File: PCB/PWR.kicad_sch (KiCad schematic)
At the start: 21 parts, among them U3 LT8610

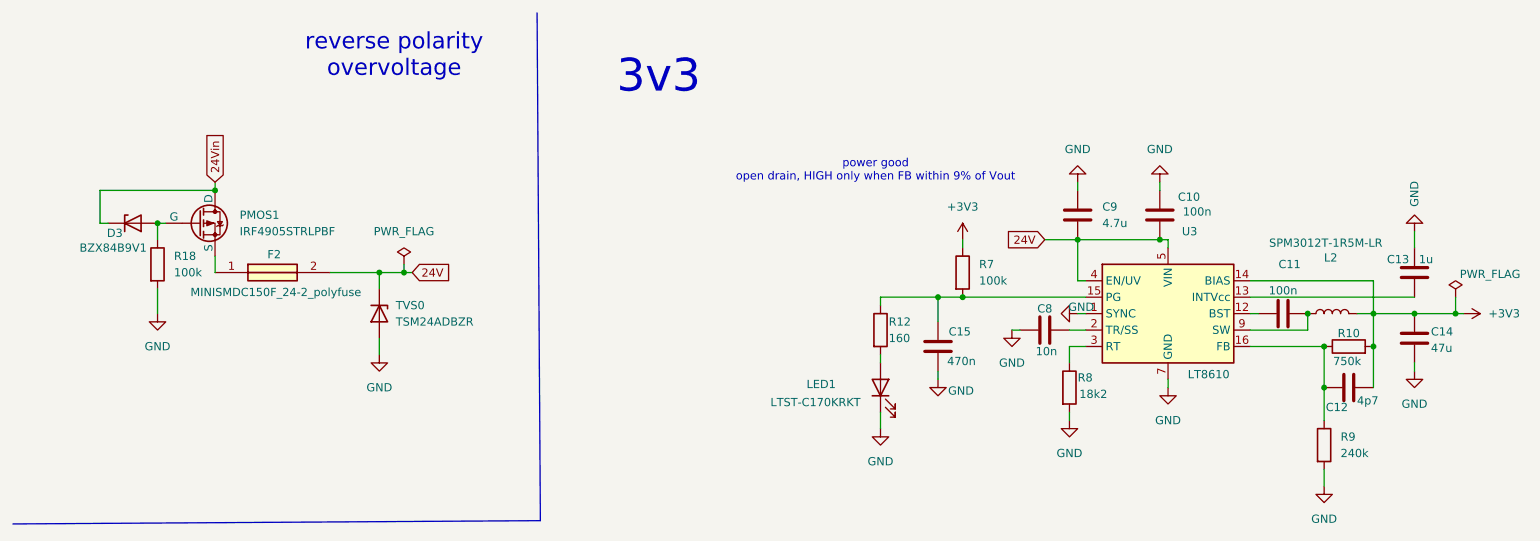
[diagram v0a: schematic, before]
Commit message: pcb version ready for final check
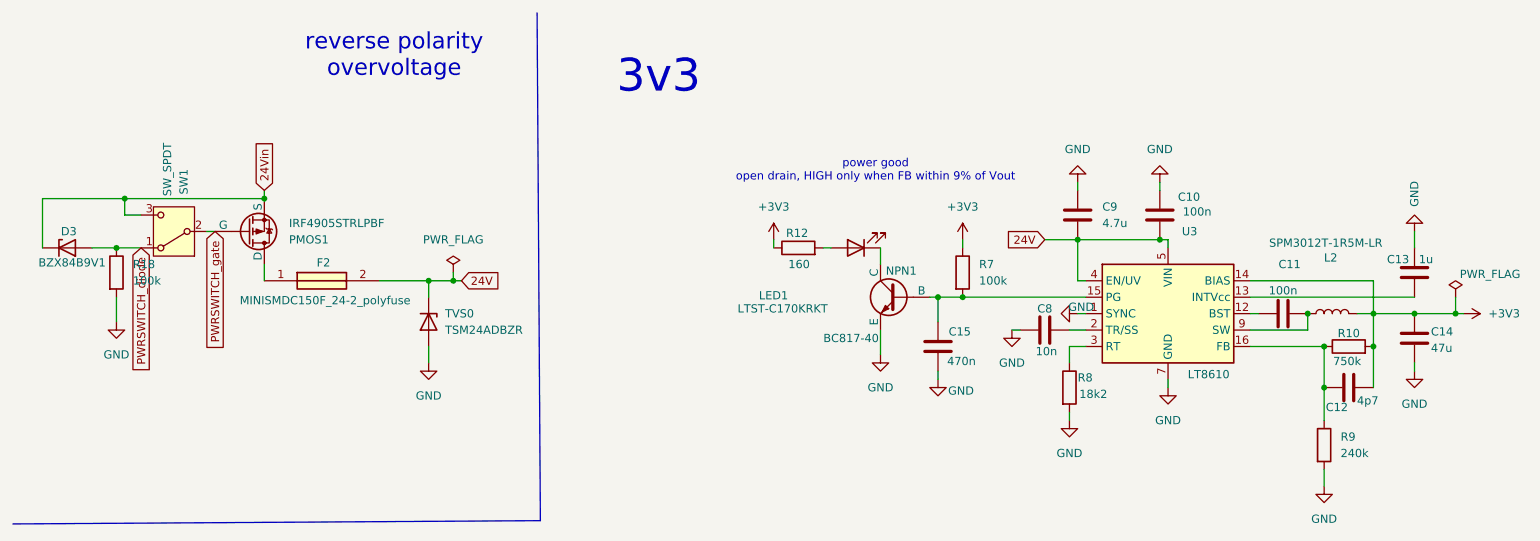
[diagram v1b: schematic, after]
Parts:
- added NPN1: BC817-40, Package_TO_SOT_SMD:TSOT-23_HandSoldering, symbol Simulation_SPICE:NPN
- added SW1: SW_SPDT, symbol Switch:SW_SPDT
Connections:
- net +3V3: now also R12.1
- net 24Vin: now also PMOS1.3 (S), SW1.3 (C); no longer PMOS1.1 (D)
- net GND: now also NPN1.3 (E); no longer LED1.1 (K)
- net PWRSWITCH_diode: now reaches D3.2 (A), R18.1
- net PWRSWITCH_diode: now also SW1.1 (A); no longer PMOS1.2 (G)
- net at C15.2, R7.2, U3.15 (PG): now also NPN1.2 (B); no longer R12.1
- net at F2.1: now also PMOS1.1 (D); no longer PMOS1.3 (S)
- new net: LED1.1 (K), NPN1.1 (C)
- new net PWRSWITCH_gate: PMOS1.2 (G), SW1.2 (B)
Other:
- moved on the sheet: D3, F2, LED1, PMOS1, R12, R18, TVS0
